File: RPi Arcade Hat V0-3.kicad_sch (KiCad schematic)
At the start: 94 parts, among them J1 Raspberry_Pi_2_3, J10 Coin/Note Input, J11 +24V IN, J12 +12V OUT, J13 Player 1, J14 Player 2, J15 Player 3, J16 Player 4, J19 Coin Counter, J2 Player 1, J3 Player 2, J4 Spares, J5 Player 3, J6 Player 4, J7 +24V OUT, J8 Counter Bypass, Q1 BC847, Q10 BC847, Q11 BC847, Q12 BC847, Q13 BC847, Q14 BC847, Q15 BC847, Q16 BC847, Q2 BC847, Q3 BC847, Q4 BC847, Q5 BC847, Q6 BC847, Q7 BC847, Q8 BC847, Q9 BC847, U1 SN74HC32N, U10 NE555DR, U12 SN74HC08N, U13 NE555DR, U14 SN74HC74N, U18 SN74HC08N, U3 LM2595S-12

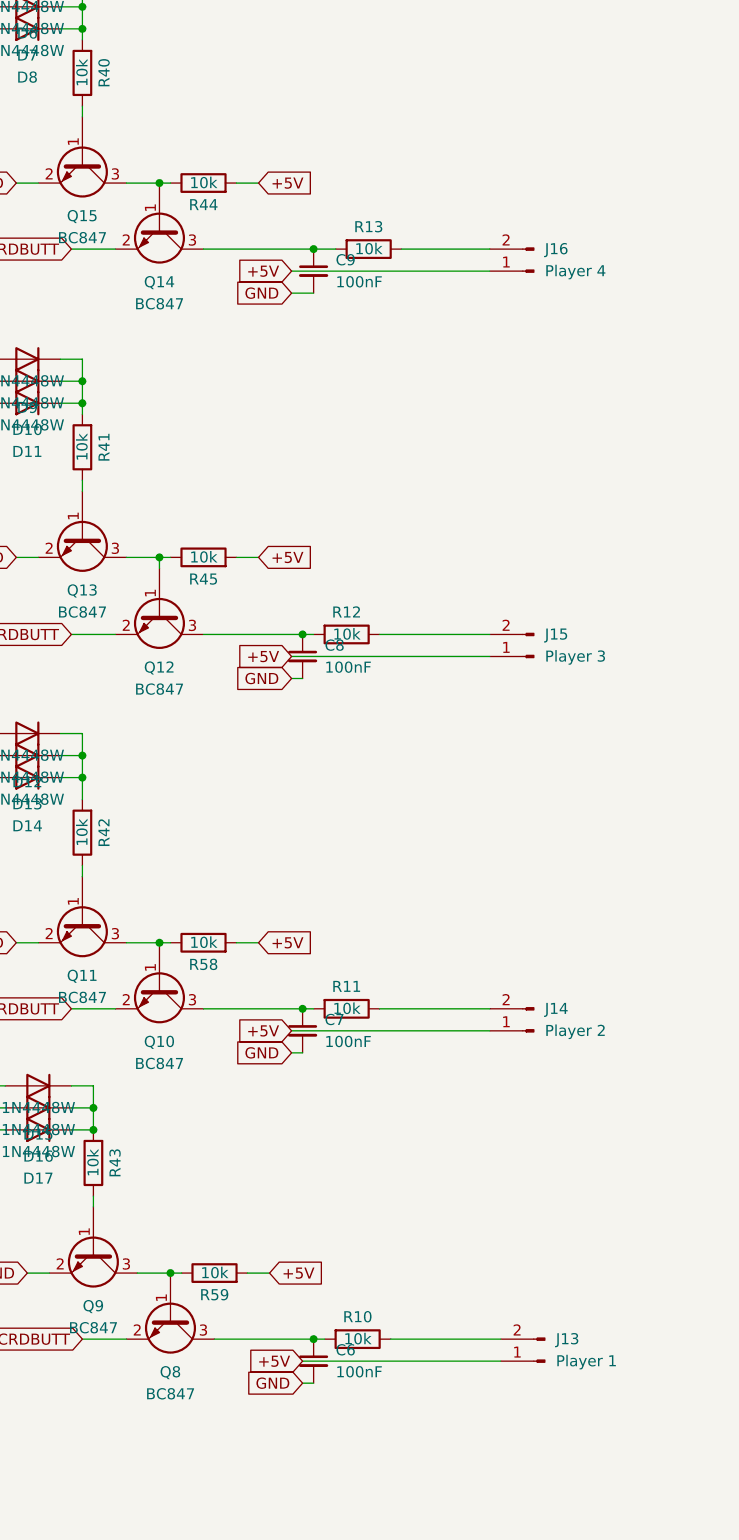
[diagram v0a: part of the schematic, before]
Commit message: Reverted Changes
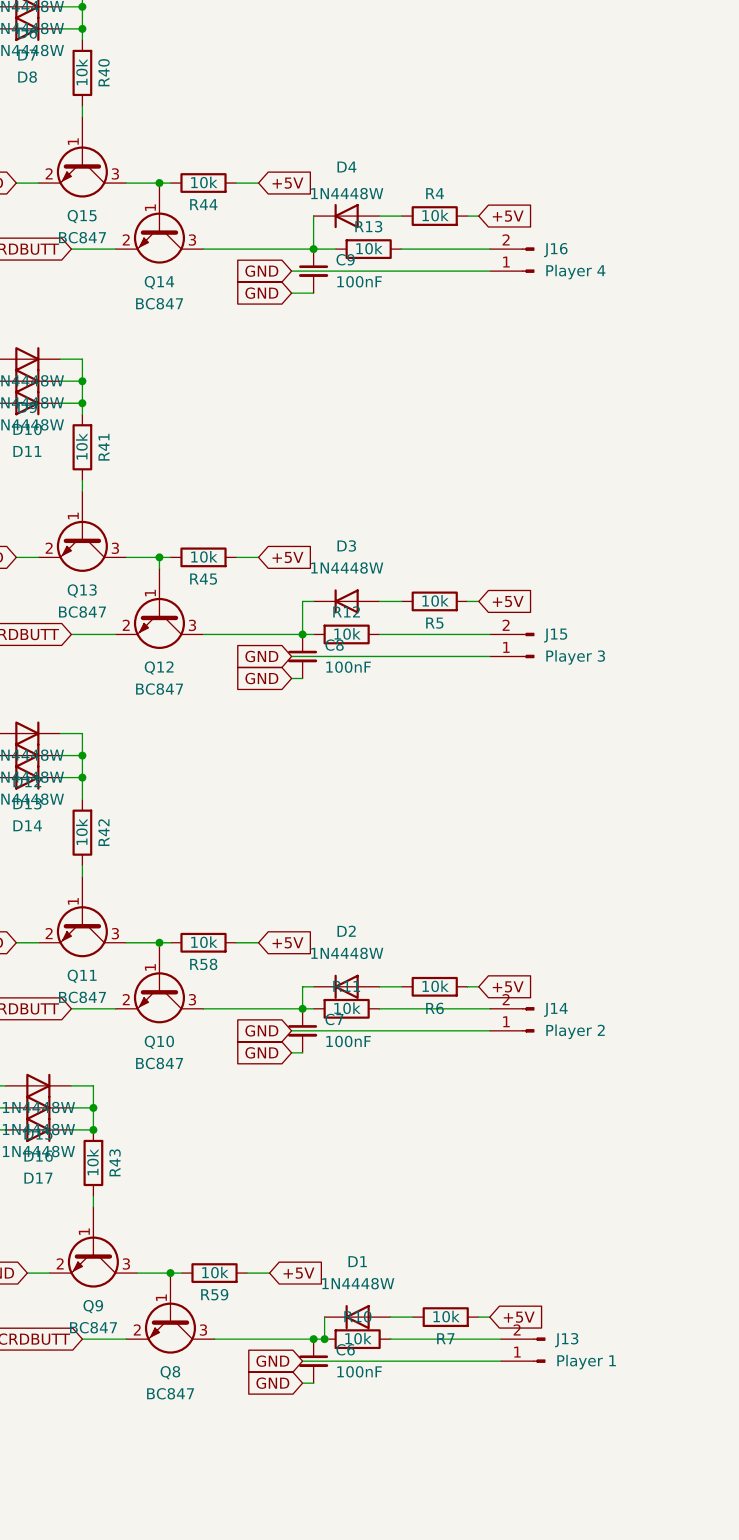
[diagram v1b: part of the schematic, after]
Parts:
- added D1, D2, D3, D4: 1N4448W, Diode_SMD:D_SOD-123, symbol Diode:1N4448W
- added R4, R5, R6, R7: 10k, Resistor_SMD:R_1206_3216Metric, symbol Device:R
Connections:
- net +5V: now also R4.2, R5.2, R6.2, R7.2; no longer J13.1 (Pin_1), J14.1 (Pin_1), J15.1 (Pin_1), J16.1 (Pin_1)
- net GND: now also J13.1 (Pin_1), J14.1 (Pin_1), J15.1 (Pin_1), J16.1 (Pin_1)
- net at C6.1, Q8.3 (C), R10.2: now also D1.1 (K)
- net at C7.1, Q10.3 (C), R11.2: now also D2.1 (K)
- net at C8.1, Q12.3 (C), R12.2: now also D3.1 (K)
- net at C9.1, Q14.3 (C), R13.2: now also D4.1 (K)
- new net: D2.2 (A), R6.1
- new net: D1.2 (A), R7.1
- new net: D3.2 (A), R5.1
- new net: D4.2 (A), R4.1
